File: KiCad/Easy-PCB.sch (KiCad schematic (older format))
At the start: 1 part, among them J3 HLW20R-2C7LF

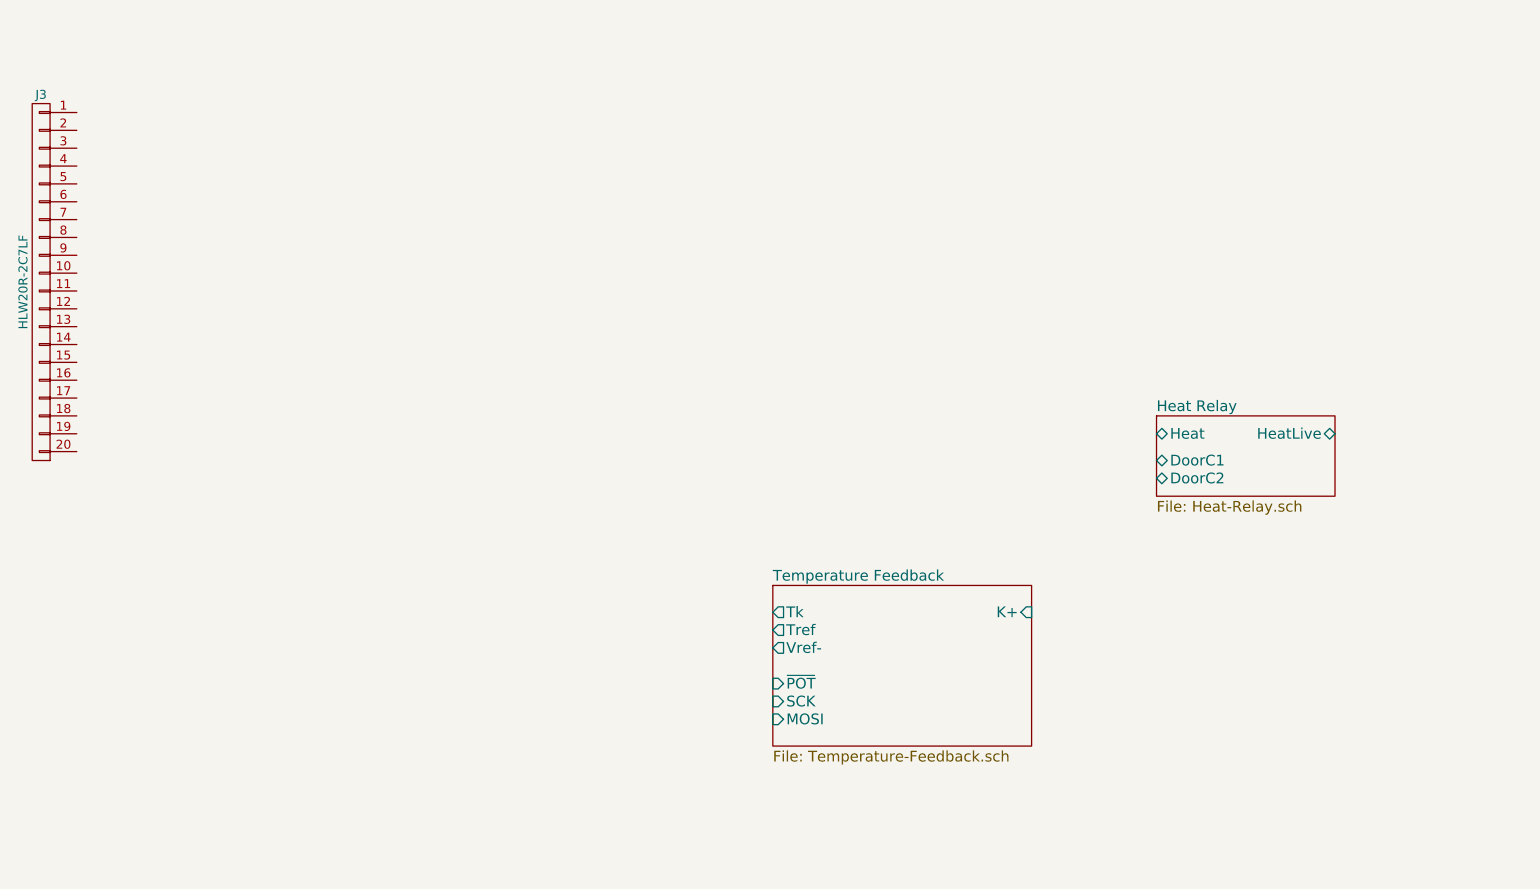
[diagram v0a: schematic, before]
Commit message: microcontroller schematic kicad
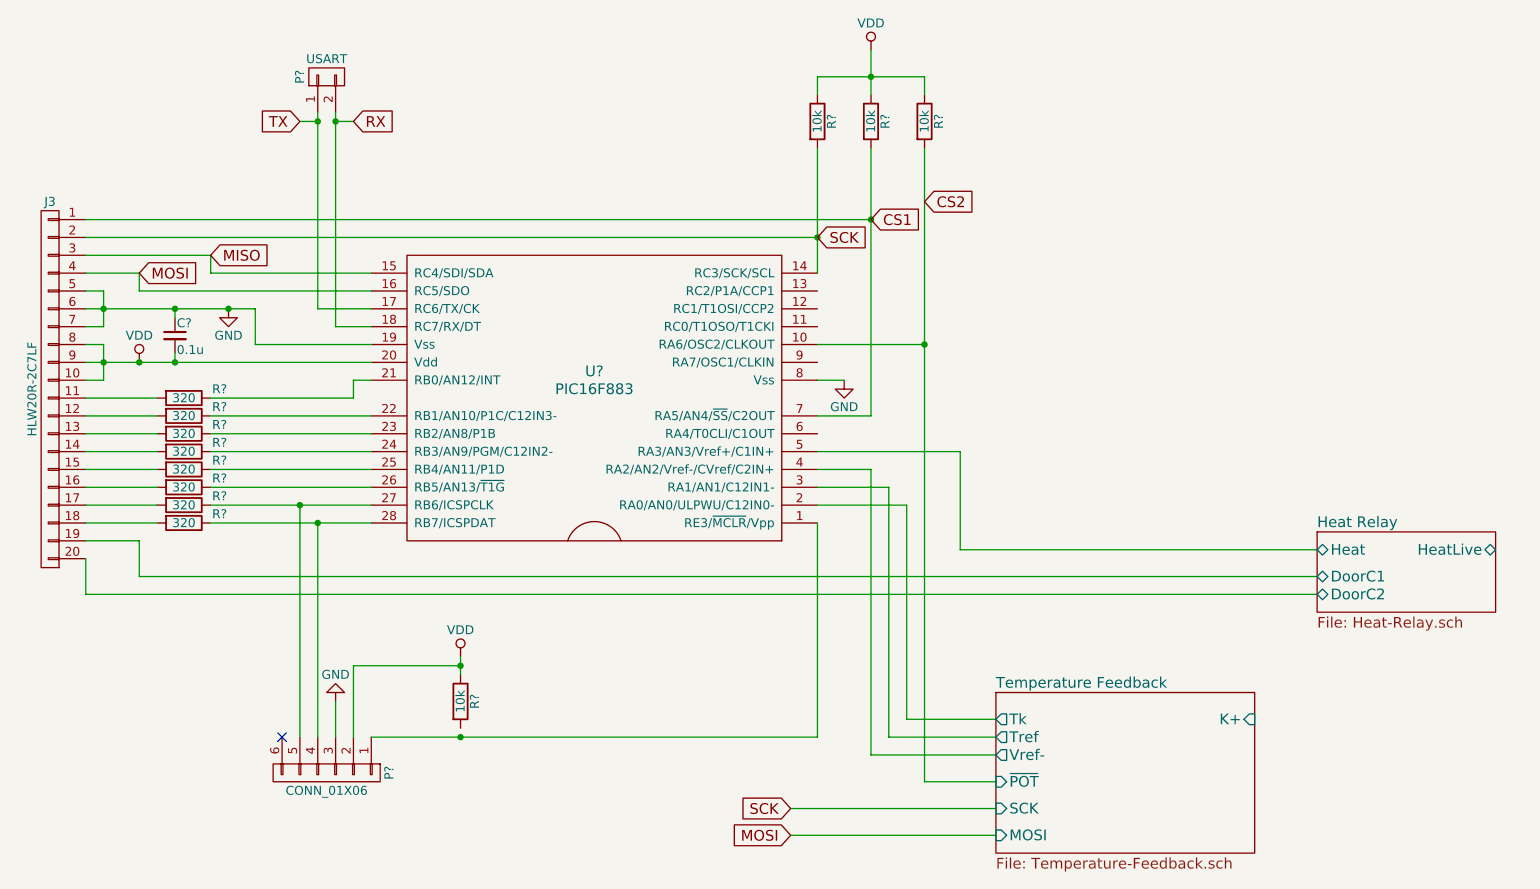
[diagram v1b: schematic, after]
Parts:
- added C?: 0.1u, symbol C_Small
- added P?: USART, symbol CONN_01X02
- added P?: CONN_01X06, symbol CONN_01X06
- added R? (x8): 320, symbol R
- added R? (x4): 10k, symbol R
- added U?: PIC16F883, symbol PIC16F883
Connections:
- net Heat Relay/DoorC1: now also J3.19 (P19)
- net Heat Relay/DoorC2: now also J3.20 (P20)
- net Heat Relay/Heat: now also U?.5 (RA3/AN3/Vref+/C1IN+)
- net Temperature Feedback/Tk: now also U?.2 (RA0/AN0/ULPWU/C12IN0-)
- net Temperature Feedback/Tref: now also U?.3 (RA1/AN1/C12IN1-)
- net Temperature Feedback/Vref-: now also U?.4 (RA2/AN2/Vref-/CVref/C2IN+)
- net CS1: now reaches J3.1 (P1)
- net CS1: now also R?.2, U?.7 (RA5/AN4/~SS~/C2OUT)
- net VDD: now reaches J3.10 (P10)
- net VDD: now also J3.8 (P8), J3.9 (P9), C?.2, P?.2 (P2), R?.1, R?.1, R?.1, R?.1, U?.20 (Vdd)
- net at J3.11 (P11): now also R?.2
- net at J3.12 (P12): now also R?.2
- net at J3.13 (P13): now also R?.2
- net at J3.14 (P14): now also R?.2
- net at J3.15 (P15): now also R?.2
- net at J3.16 (P16): now also R?.2
- net at J3.17 (P17): now also R?.2
- net at J3.18 (P18): now also R?.2
- net SCK: now reaches J3.2 (P2)
- net SCK: now also R?.2, U?.14 (RC3/SCK/SCL)
- net MISO: now reaches J3.3 (P3)
- net MISO: now also U?.15 (RC4/SDI/SDA)
- net MOSI: now reaches J3.4 (P4)
- net MOSI: now also U?.16 (RC5/SDO)
- net GND: now reaches J3.5 (P5)
- net GND: now also J3.6 (P6), J3.7 (P7), C?.1, P?.3 (P3), U?.19 (Vss), U?.8 (Vss)
- new net: P?.1 (P1), U?.1 (RE3/~MCLR~/Vpp)
- new net: R?.1, U?.21 (RB0/AN12/INT)
- new net: R?.1, U?.22 (RB1/AN10/P1C/C12IN3-)
- new net: R?.1, U?.23 (RB2/AN8/P1B)
- new net: R?.1, U?.24 (RB3/AN9/PGM/C12IN2-)
- new net: R?.1, U?.25 (RB4/AN11/P1D)
- new net: R?.1, U?.26 (RB5/AN13/~T1G)
- new net: P?.5 (P5), R?.1, U?.27 (RB6/ICSPCLK)
- new net: P?.4 (P4), R?.1, U?.28 (RB7/ICSPDAT)
- new net CS2: R?.2, U?.10 (RA6/OSC2/CLKOUT)
- new net RX: P?.2 (P2), U?.18 (RC7/RX/DT)
- new net TX: P?.1 (P1), U?.17 (RC6/TX/CK)
- no-connect marks 0 -> 1
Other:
- moved on the sheet: J3
